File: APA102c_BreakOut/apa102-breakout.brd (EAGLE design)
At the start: 76.8 x 51.4 mm, 52 parts

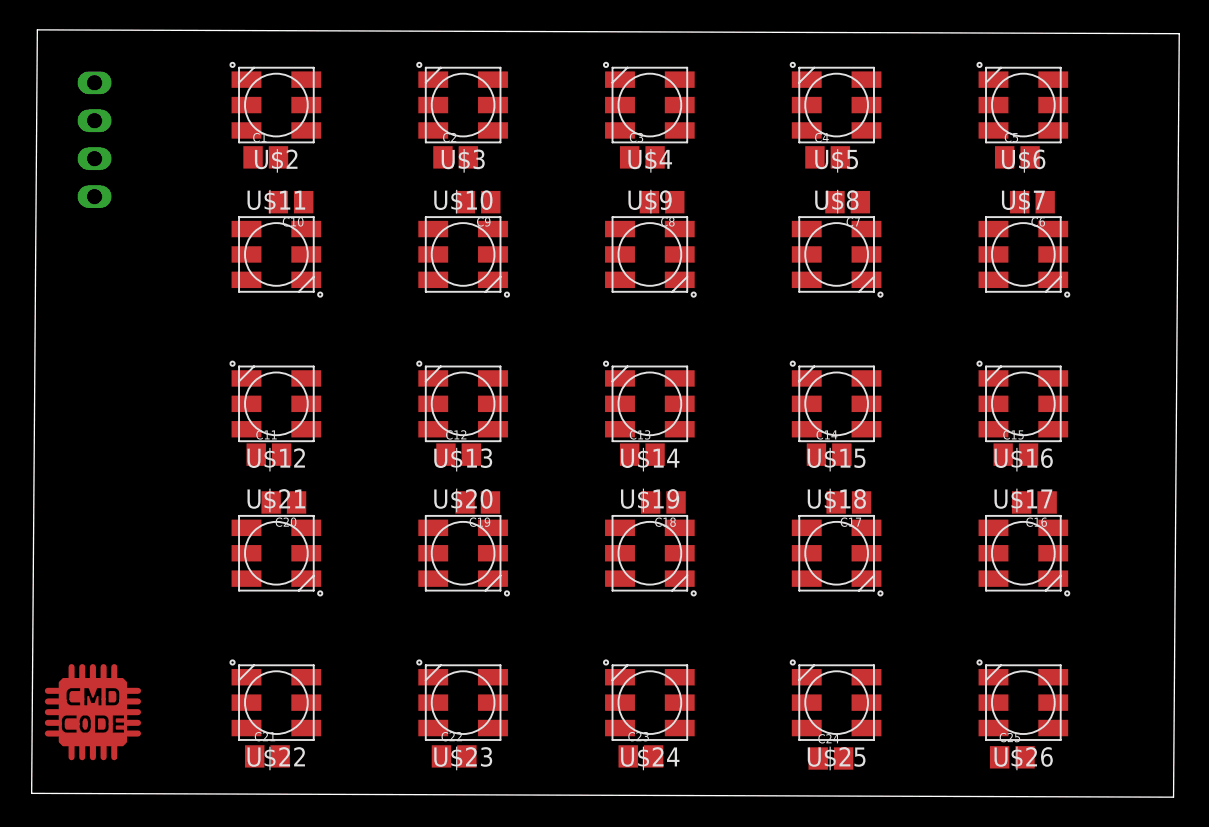
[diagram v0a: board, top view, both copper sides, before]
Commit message: updated routing again
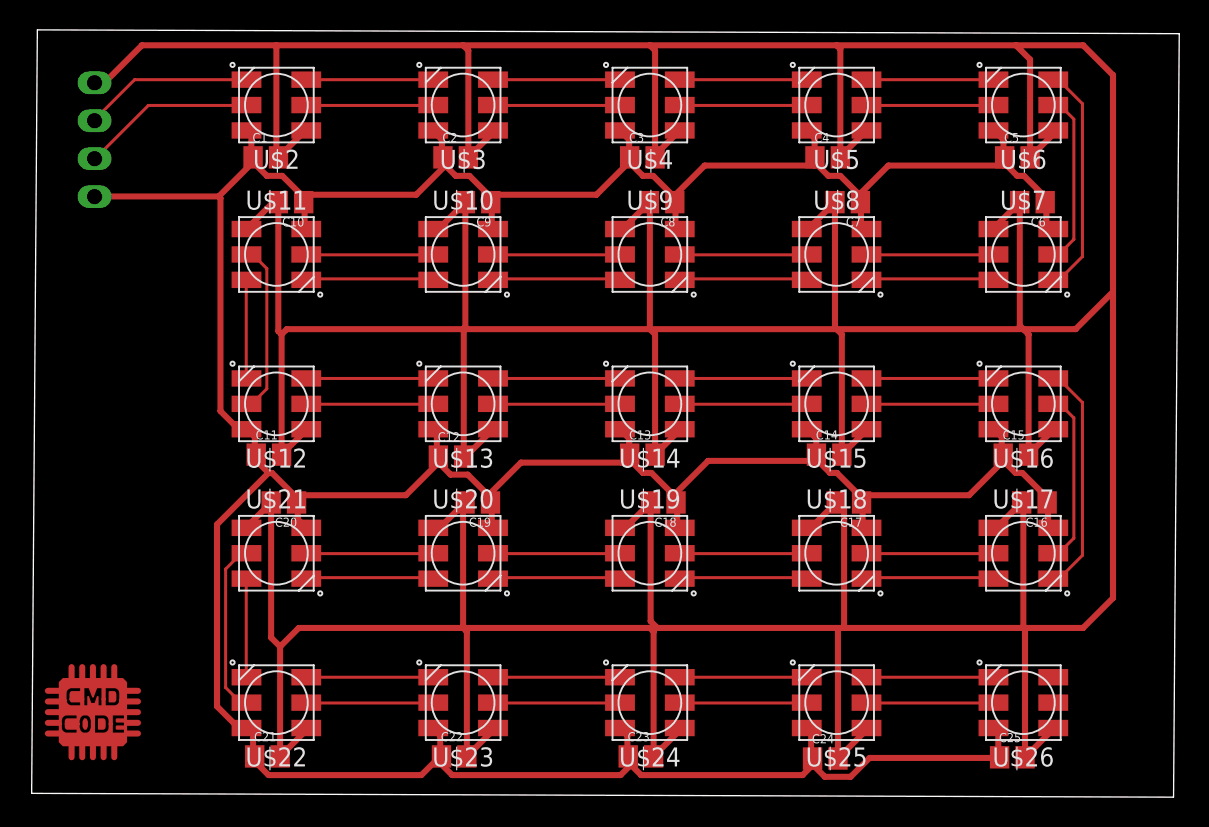
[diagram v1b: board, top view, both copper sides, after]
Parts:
- moved C12 0.52 mm to (28.2, 22.5)
- moved C24 0.38 mm to (53.2, 2.26)
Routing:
- net VCC: track 0.00 -> 494.1 mm
- net GND: track 0.00 -> 291.1 mm
- net N$61: track 0.00 -> 15.5 mm
- net N$41: track 0.00 -> 15.5 mm
- net N$62: track 0.00 -> 11.7 mm
- net N$42: track 0.00 -> 11.7 mm
- net CLK: track 0.00 -> 11.7 mm
- net N$73: track 0.00 -> 11.6 mm
- net N$51: track 0.00 -> 11.6 mm
- net DATA: track 0.00 -> 11.3 mm
- net N$71: track 0.00 -> 8.58 mm
- net N$50: track 0.00 -> 8.58 mm
- net N$64: track 0.00 -> 8.57 mm
- net N$43: track 0.00 -> 8.57 mm
- net N$69: track 0.00 -> 8.57 mm
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
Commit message: added silk screen
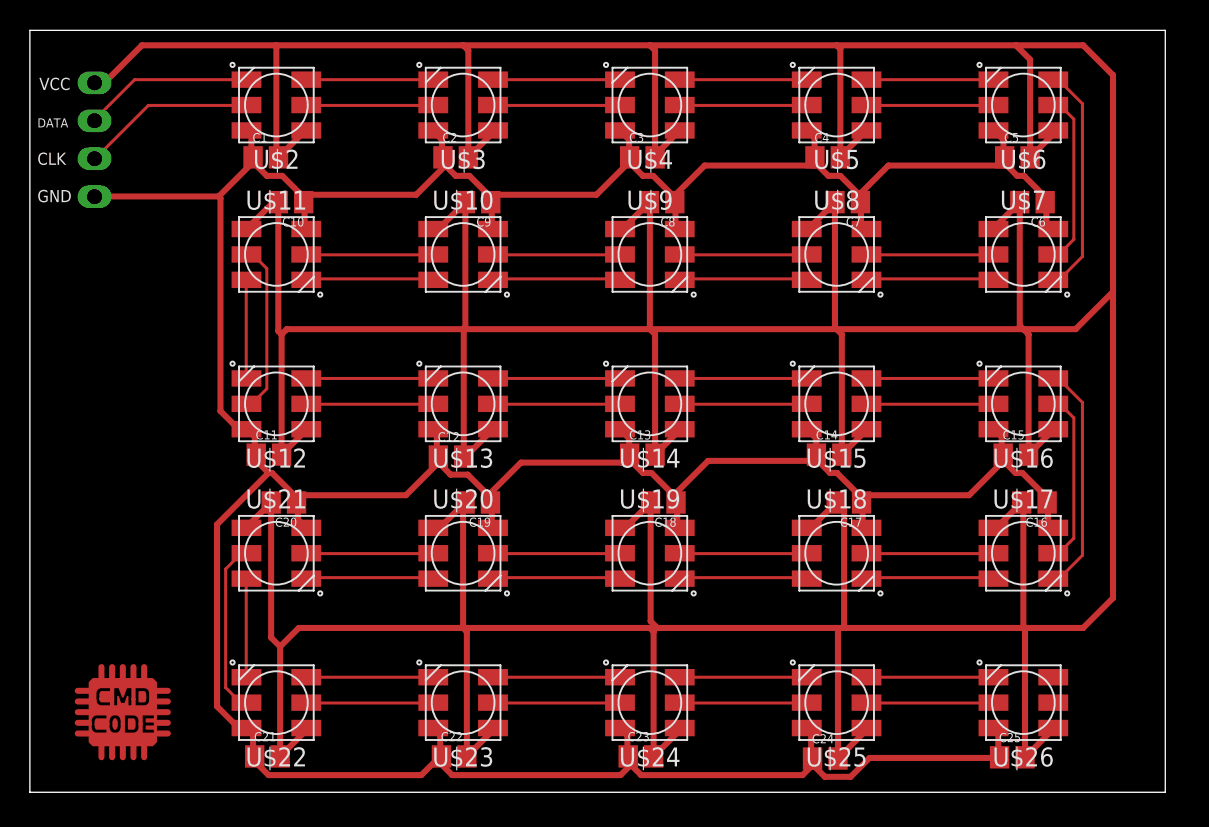
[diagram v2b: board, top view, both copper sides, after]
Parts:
- moved U$1 2.00 mm to (6.22, 5.68)
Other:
- board size 76.8 x 51.4 mm -> 76 x 51 mm
- board text added: "CLK"
- board text added: "DATA"
- board text added: "GND"
- board text added: "VCC"
